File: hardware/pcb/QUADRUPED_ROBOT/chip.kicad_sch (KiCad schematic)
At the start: 60 parts, among them J1 Conn_01x03_Socket, J2 Conn_01x04_Pin, J8 Conn_01x06_Pin, Q2 BC847, Q3 BC847, SW1 SW_Push, U2 STM32F723ZETx, Y1 25MHz

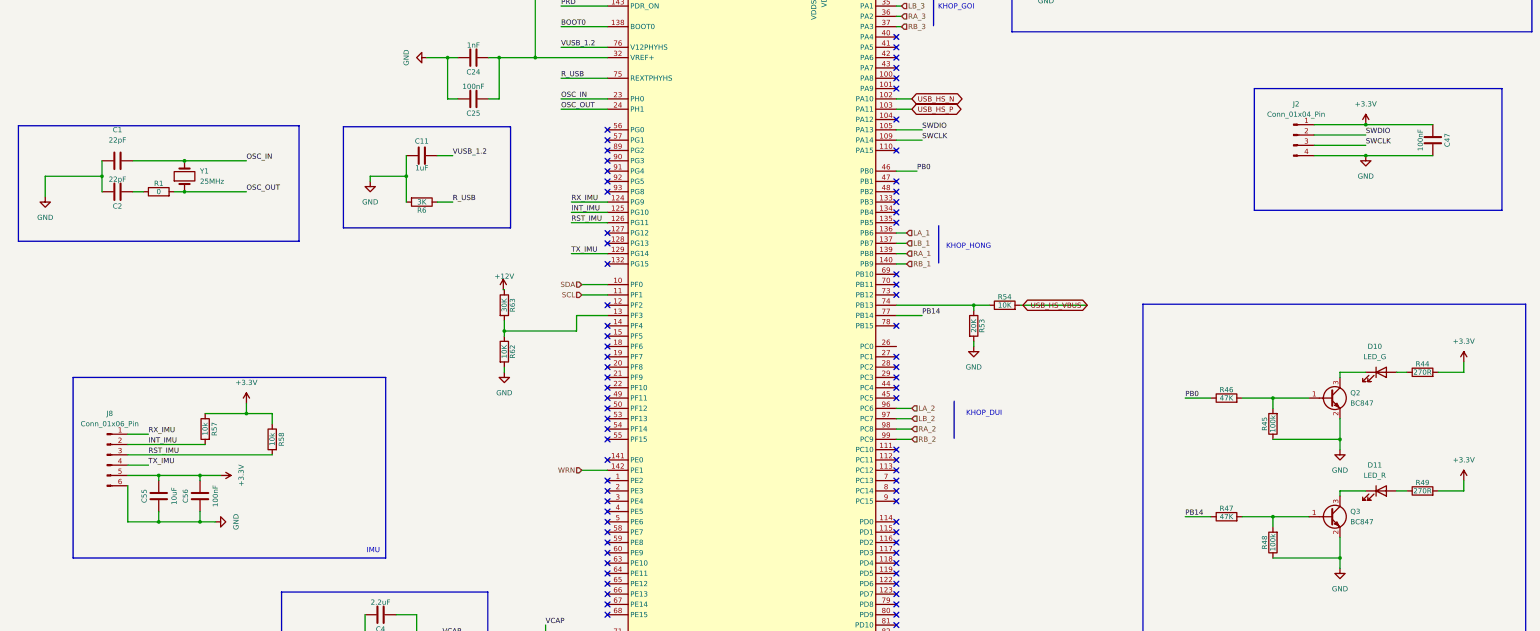
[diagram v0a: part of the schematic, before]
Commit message: :bom
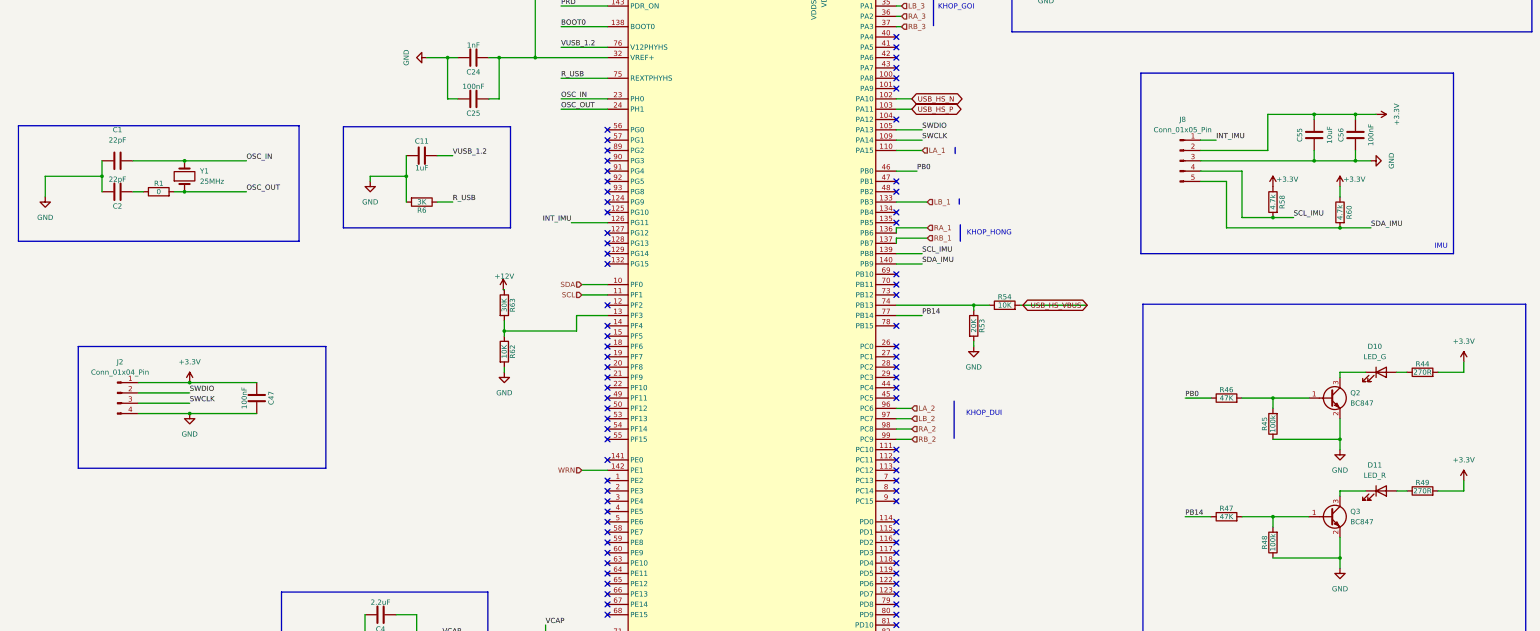
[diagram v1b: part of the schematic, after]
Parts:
- removed J8: Conn_01x06_Pin, Connector_PinSocket_2.54mm:PinSocket_1x06_P2.54mm_Vertical, symbol Connector:Conn_01x06_Pin
- removed R57: 10k, Resistor_SMD:R_0805_2012Metric, symbol Device:R
- added J8: Conn_01x05_Pin, Connector_PinSocket_2.54mm:PinSocket_1x05_P2.54mm_Vertical, symbol Connector:Conn_01x05_Pin
- added R60: 4.7k, Resistor_SMD:R_0805_2012Metric, symbol Device:R
- R58: value 10k -> 4.7k
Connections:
- net +3.3V: now also J8.2 (Pin_2), R60.1
- net GND: now also J8.3 (Pin_3)
- net INT_IMU: now also U2.126 (PG11), J8.1 (Pin_1); no longer U2.125 (PG10)
- net LA_1: now also U2.110 (PA15); no longer U2.136 (PB6)
- net LB_1: now also U2.133 (PB3); no longer U2.137 (PB7)
- net RA_1: now also U2.136 (PB6); no longer U2.139 (PB8)
- net RB_1: now also U2.137 (PB7); no longer U2.140 (PB9)
- net RST_IMU renamed SCL_IMU
- net SCL_IMU: now also U2.139 (PB8), J8.4 (Pin_4); no longer U2.126 (PG11)
- net RX_IMU: no longer names the net of U2.124 (PG9)
- net TX_IMU: no longer names the net of U2.129 (PG14)
- new net SDA_IMU: J8.5 (Pin_5), R60.2, U2.140 (PB9)
- no-connect marks 82 -> 84
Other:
- moved on the sheet: C47, C55, C56, J2
